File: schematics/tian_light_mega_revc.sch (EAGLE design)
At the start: 34 parts, among them IC2 MC33269ST-3.3T3, Q201 BUZ11

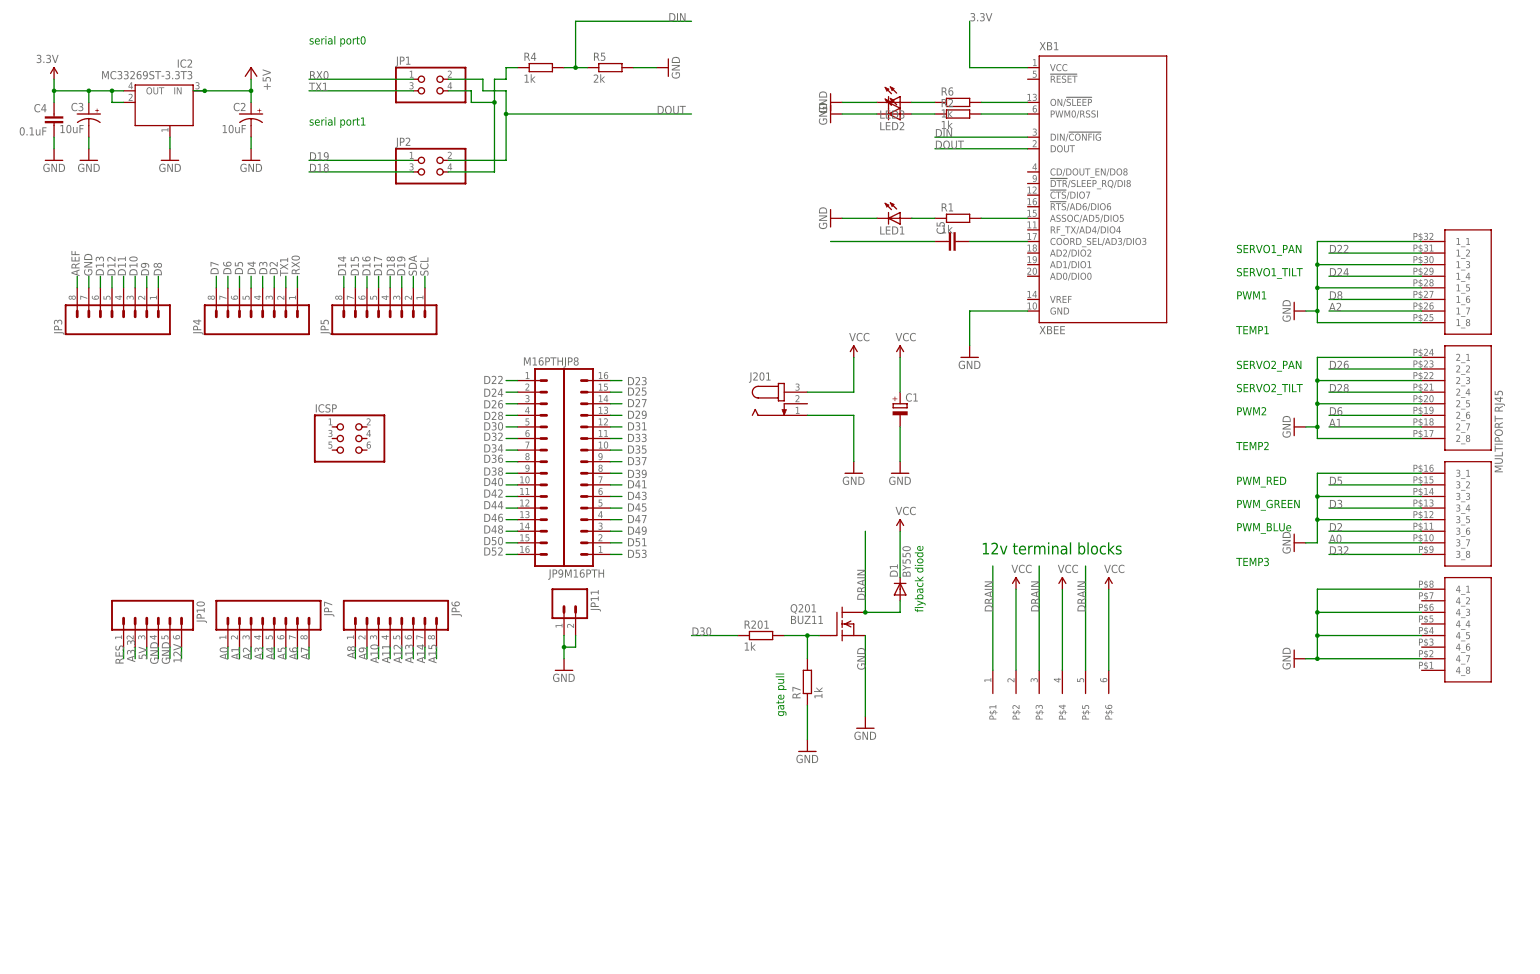
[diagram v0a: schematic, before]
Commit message: -a
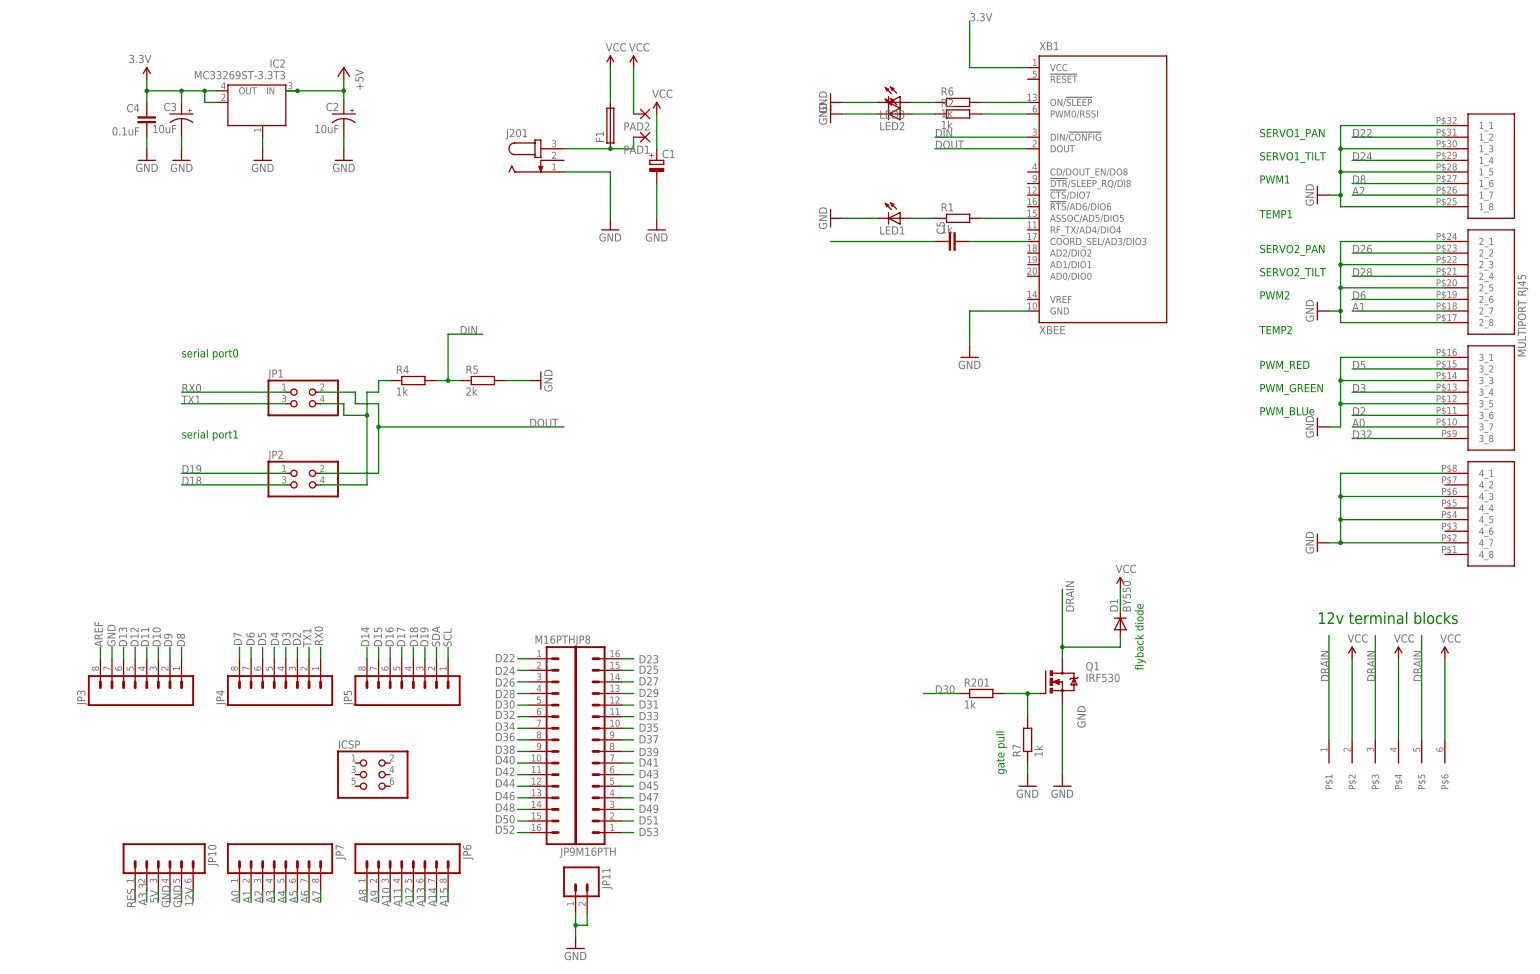
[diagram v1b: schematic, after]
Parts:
- removed Q201: BUZ11, transistor-fet:BUZ11
- added F1: (no value), fuse:SH22,5
- added PAD1, PAD2: (no value), wirepad:2,15/1,0
- added Q1: IRF530, transistor-power:IRF530
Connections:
- new net N$10: F1.1, J201.3, PAD1.P
- net 12V: now also F1.2, PAD2.P; no longer J201.3
- net DRAIN: now also Q1.D; no longer Q201.D
- net GND: now also Q1.S; no longer Q201.S
- net N$3: now also Q1.G; no longer Q201.G
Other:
- note removed: "TEMP3"
- moved on the sheet: C1, C2, C3, C4, D1, IC2, ICSP, J201, JP1, JP10, JP11, JP2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
